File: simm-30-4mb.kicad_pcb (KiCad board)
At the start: 4 copper layers, 77.7 x 19 mm, 8 parts, among them J2 Conn_01x30, U1 511400, U2 511400

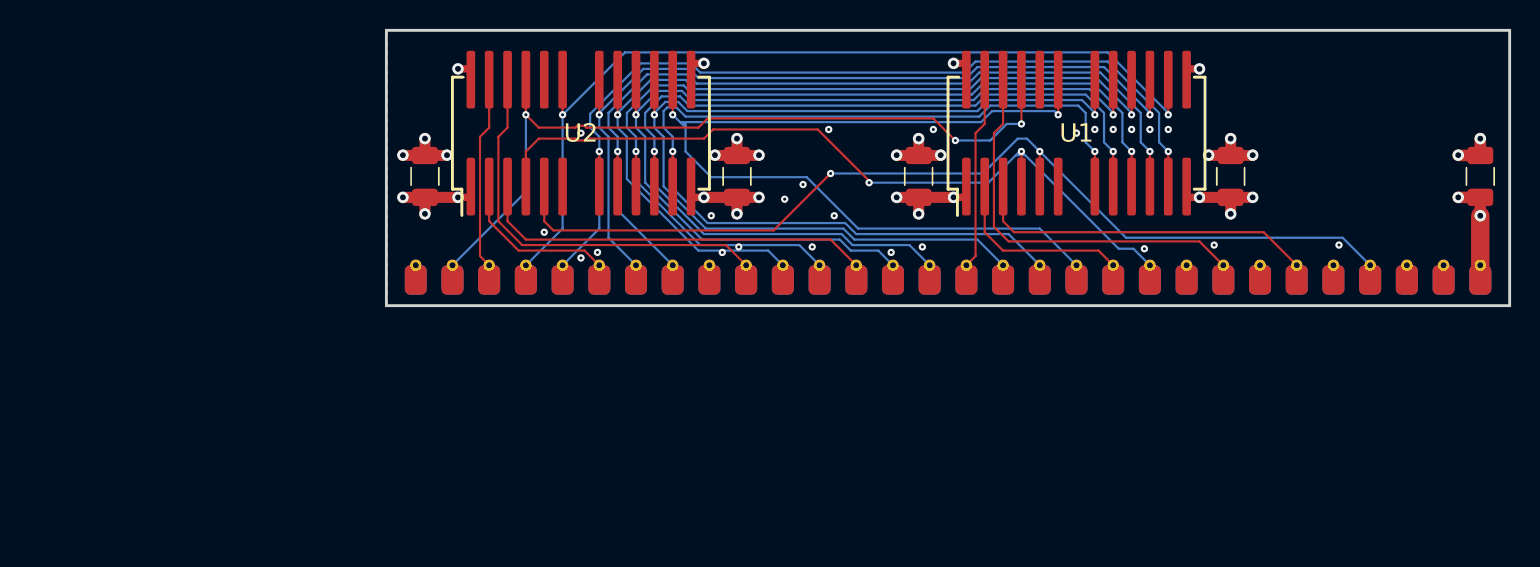
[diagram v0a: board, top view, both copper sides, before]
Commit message: Submitted to JLCPCB
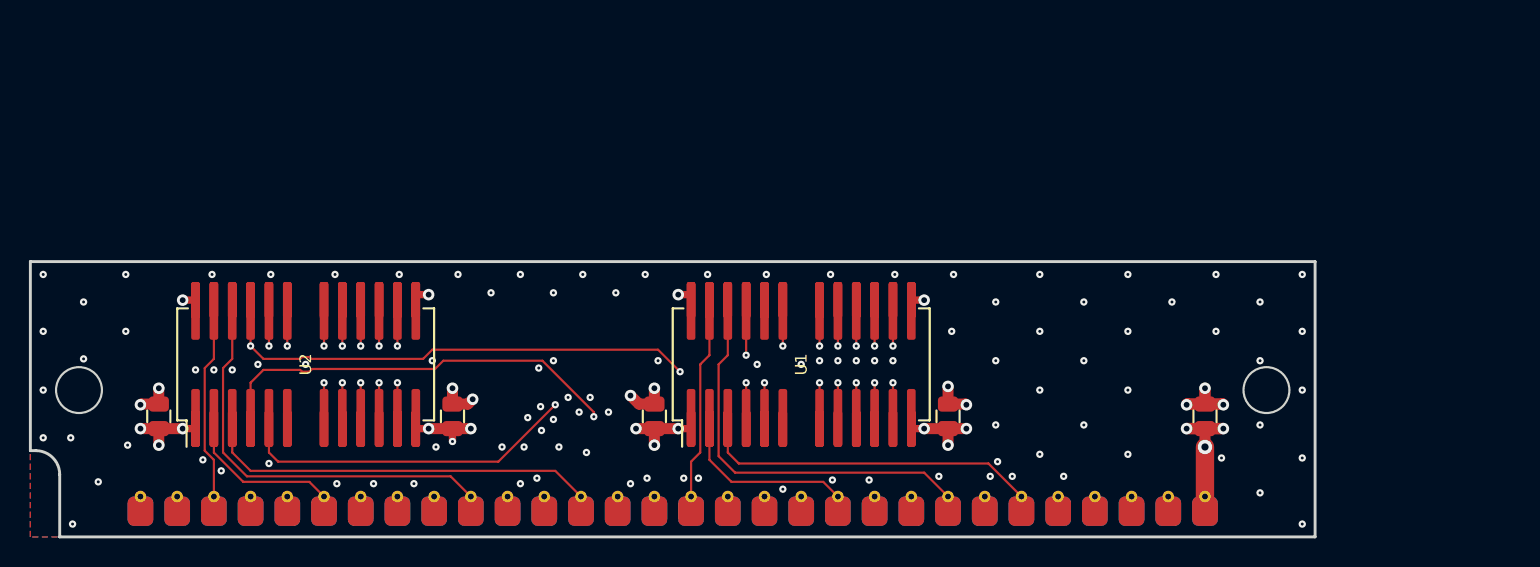
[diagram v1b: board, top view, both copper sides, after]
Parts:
- removed the C3 at (137.7, 76.7)
- removed the C3 at (159.3, 76.7)
- removed J2: Conn_01x30, stdpads:Memory_SIMM_30
- added C3: 100n, stdpads:C_0805, F.Cu at (119.4, 93.3)
- added C5: 100n, stdpads:C_0805, F.Cu at (157.5, 93.3)
- added J1: Conn_01x30, stdpads:SIMM-30_Edge, F.Cu at (120.7, 99.8)
- C1, C2, C4: footprint stdpads:C_1206 -> stdpads:C_0805
- U1, U2: value 511400 -> AS4C4M4; footprint stdpads:SOJ-24-26-300mil -> stdpads:SOP-24-26-300mil
- moved C4 40.4 mm to (139.7, 93.3)
- moved C2 25.8 mm to (105.4, 93.3)
- moved U1 24.9 mm to (129.5, 89.7)
- moved U2 24.9 mm to (95.2, 89.7)
- moved C1 24.8 mm to (85.1, 93.3)
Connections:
- U1 pad 6: Net-(U1-Pad6) -> (no net)
- U2 pad 6: Net-(U2-Pad6) -> (no net)
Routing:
- net GND: track 25.3 -> 22.3 mm, vias 42 -> 121
- net +5V: track 29.6 -> 26.8 mm, vias 14 -> 15
- net /~WE~: track 57.0 -> 57.6 mm
- added copper zone on B.Cu, net +5V
- added copper zone on In2.Cu, net GND
- removed copper zone on In2.Cu, net +5V
- removed copper zone on B.Cu, net GND
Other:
- board size 77.7 x 19 mm -> 88.9 x 19 mm
- rule solder_mask_min_width: 0.1524 -> 0.127
- board text added: "4 MB RAM"
- board text added: "4190A"
- board text added: "GW"
- board text added: "Garrett’s Workshop"
- board text added: "JLCJLCJLC"
